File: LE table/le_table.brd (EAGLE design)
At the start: 200 x 20 mm, 59 parts, among them CON2 CONNECTOR, CON3 PINHEAD_1X09-2, CON4 PINHEAD_1X09-2, CON5 CONNECTOR, IC1 LM2902DT, IC2 CD4066, IC3 M74HCT74, Q1 PHOTOTRANSISTOR-3MM, Q2 PHOTOTRANSISTOR-0805, Q3 PHOTOTRANSISTOR-3MM, Q4 PHOTOTRANSISTOR-0805, Q5 PHOTOTRANSISTOR-3MM, Q6 PHOTOTRANSISTOR-0805, Q7 PHOTOTRANSISTOR-3MM, Q8 PHOTOTRANSISTOR-0805, Q9 IRLML2502-SOT23

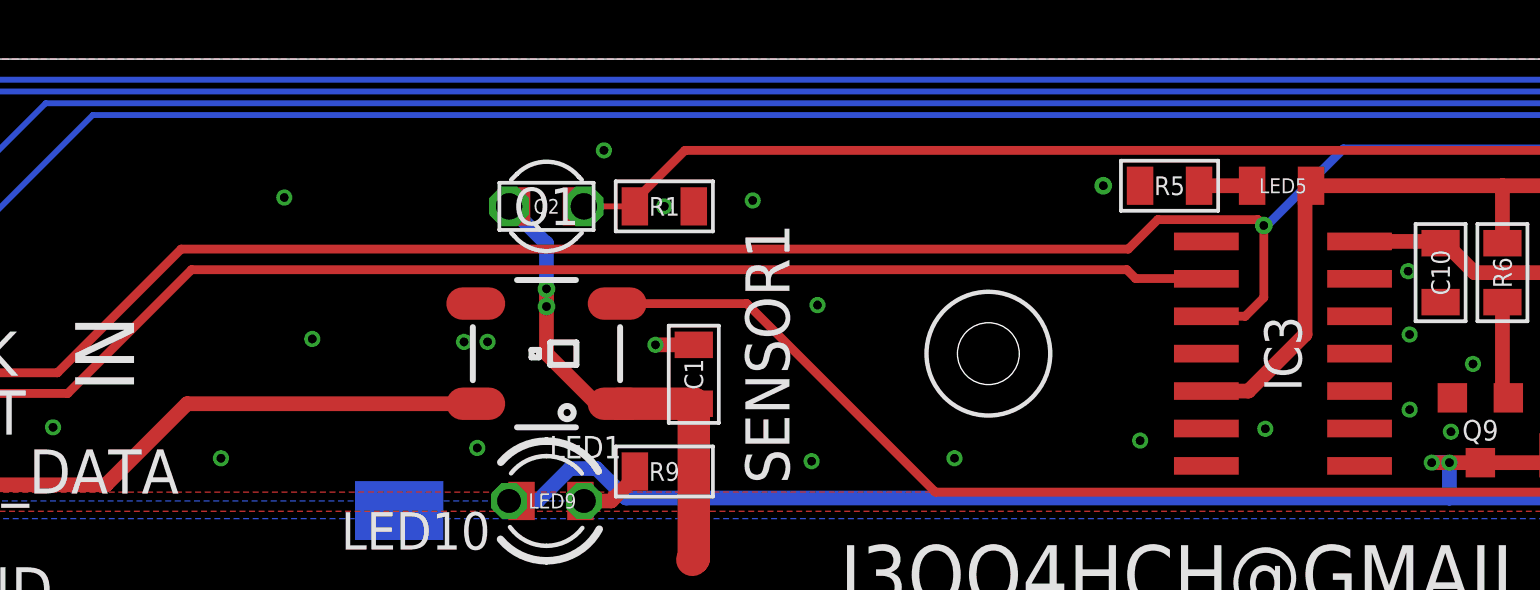
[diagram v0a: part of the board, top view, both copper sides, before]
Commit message: Software import
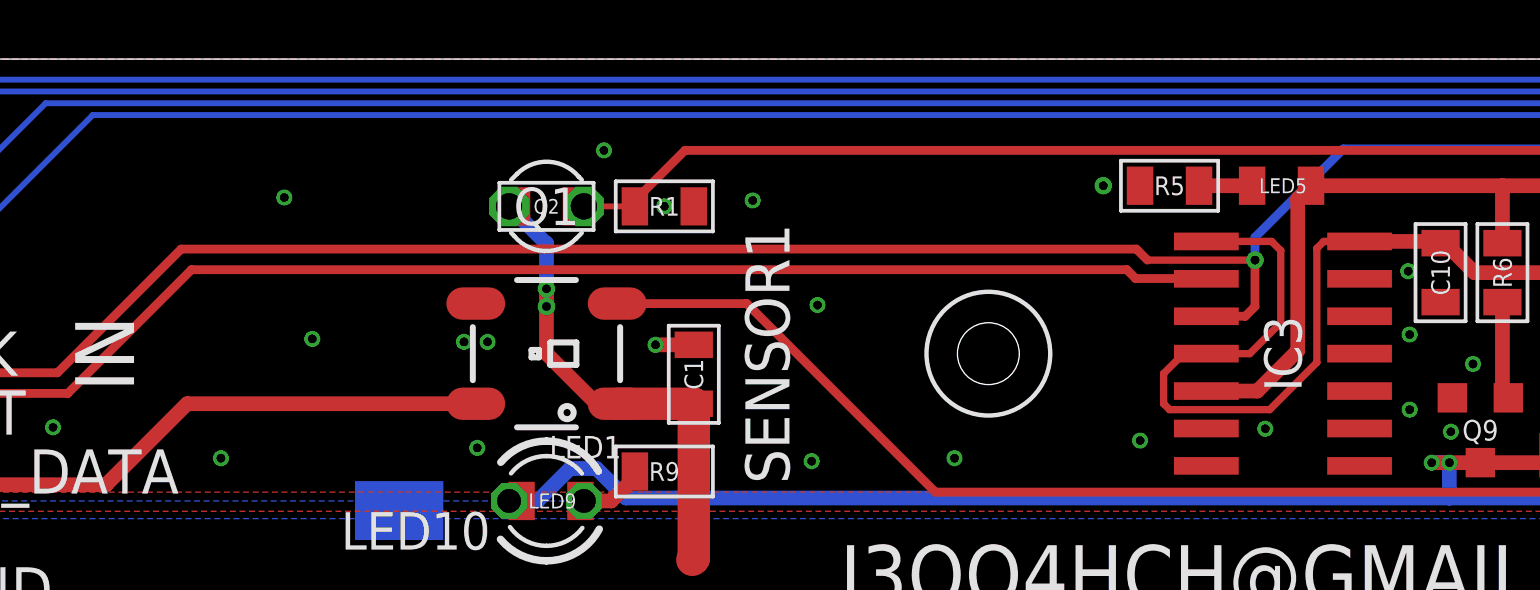
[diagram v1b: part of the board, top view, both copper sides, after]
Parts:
- R1, R2, R3, R4: value 2K -> 15-20K
- R10, R11, R12, R9: value 240R -> 150R
- R6: value 2K -> 150R
- RN2: value (none) -> 150R
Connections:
- net VDD_5V: now also IC3.1, IC3.4
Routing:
- net VDD_5V: track 111.7 -> 133.9 mm
- net CLK: track 207.9 -> 207.2 mm
